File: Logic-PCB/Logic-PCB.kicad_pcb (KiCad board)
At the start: 2 copper layers, 140 parts, among them IC1 74LVC1G74DC-Q100H, IC10 SN74LVC1G11MDCKREP, IC11 SN74LVC1G11MDCKREP, IC12 SN74LVC1G97QDBVRQ1, IC14 TMUX1208QRSVRQ1, IC15 TMUX1208QRSVRQ1, IC16 TMUX1208QRSVRQ1, IC17 TMUX1208QRSVRQ1, IC18 TMUX1208QRSVRQ1, IC19 TMUX1208QRSVRQ1, IC2 74HC73D,653, IC20 TMUX1208QRSVRQ1, IC21 TMUX1208QRSVRQ1, IC22 TMUX1208QRSVRQ1, IC23 NCV4274CDT33RKG, IC3 SN74LVC1G02DBVR, IC4 SN74LVC1G02DBVR, IC6 74AUP1T87GWH, IC7 74HC73D,653, IC8 TLC555QDRQ1, IC9 74HC73D,653, J1 CX70M-24P1, Q1 MMBT2222, Q10 MMBT2907A-7-F, Q11 MMBT2222, Q12 MMBT2222, Q13 MMBT2907A-7-F, Q2 MMBT2222, Q3 MMBT2222, Q4 MMBT2222, Q5 MMBT2907A-7-F, Q6 MMBT2907A-7-F, Q7 MMBT2222, Q8 MMBT2222, Q9 MMBT2907A-7-F, SW1 SW_Push, SW2 SW_Push, U1 74AHC1G86W5-7, U2 BAT-HLD-001-TR, U3 NC7S08M5X

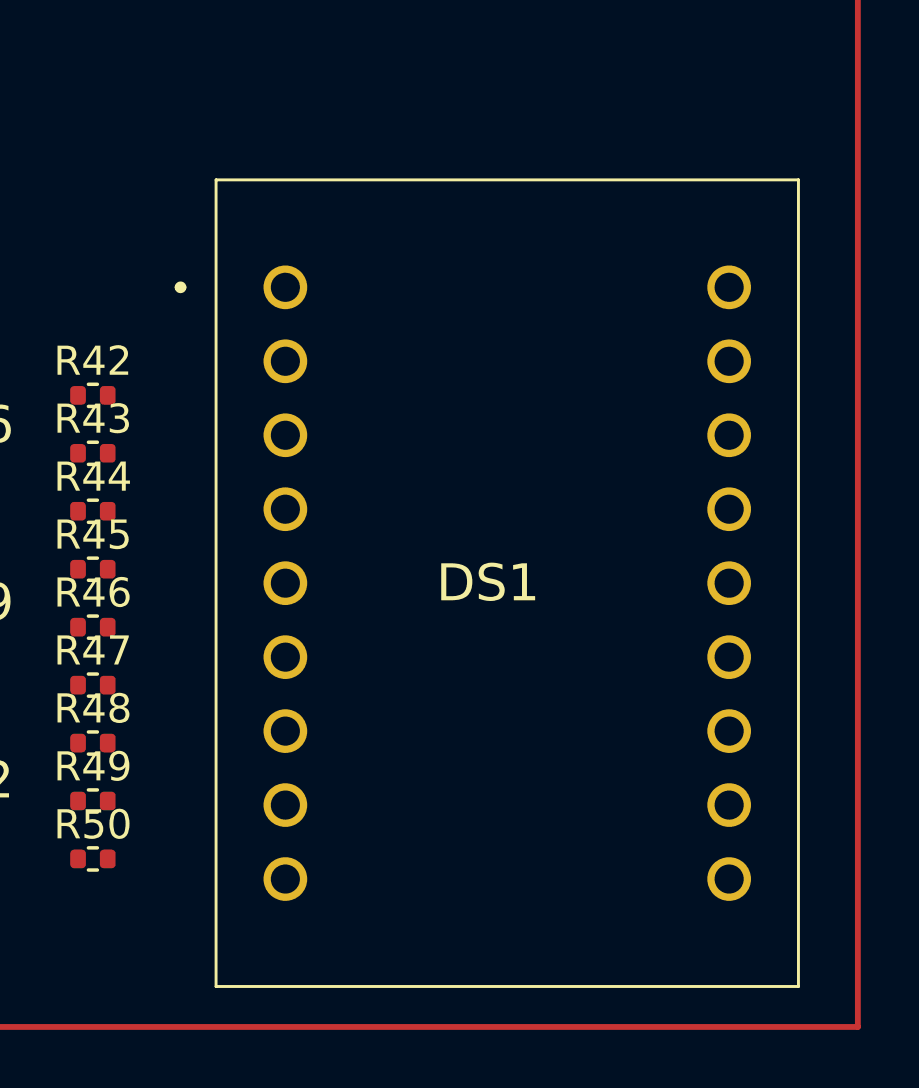
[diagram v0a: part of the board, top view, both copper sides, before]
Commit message: CMOS
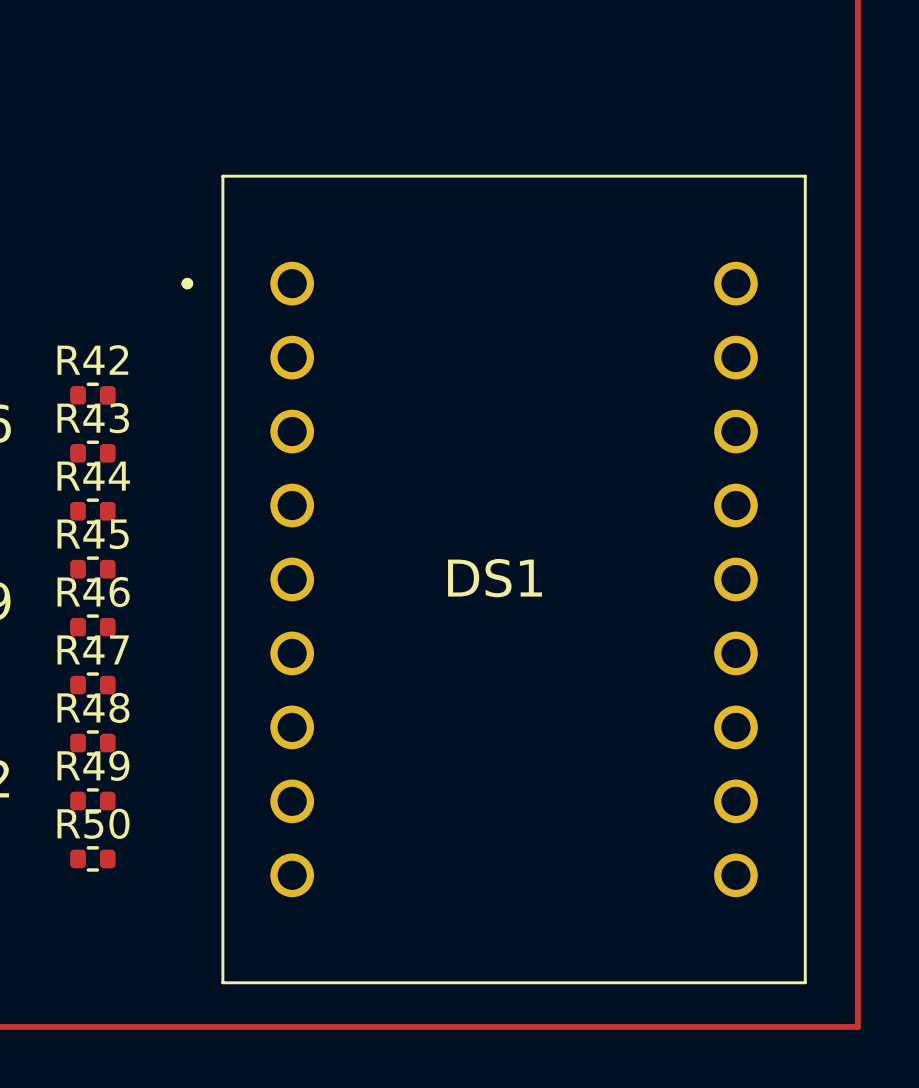
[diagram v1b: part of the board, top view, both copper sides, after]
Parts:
- moved DS1 0.27 mm to (139.3, 129.4)
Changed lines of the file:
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@@
   )
   (footprint "SamacSys_Parts:PSA0811GWA" (layer "F.Cu")
-    (at 139.11 129.54)
+    (at 139.344 129.413)
     (descr "PSA08-11GWA-1")
     (tags "Display")
